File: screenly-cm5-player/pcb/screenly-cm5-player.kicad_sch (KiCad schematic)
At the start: 0 parts

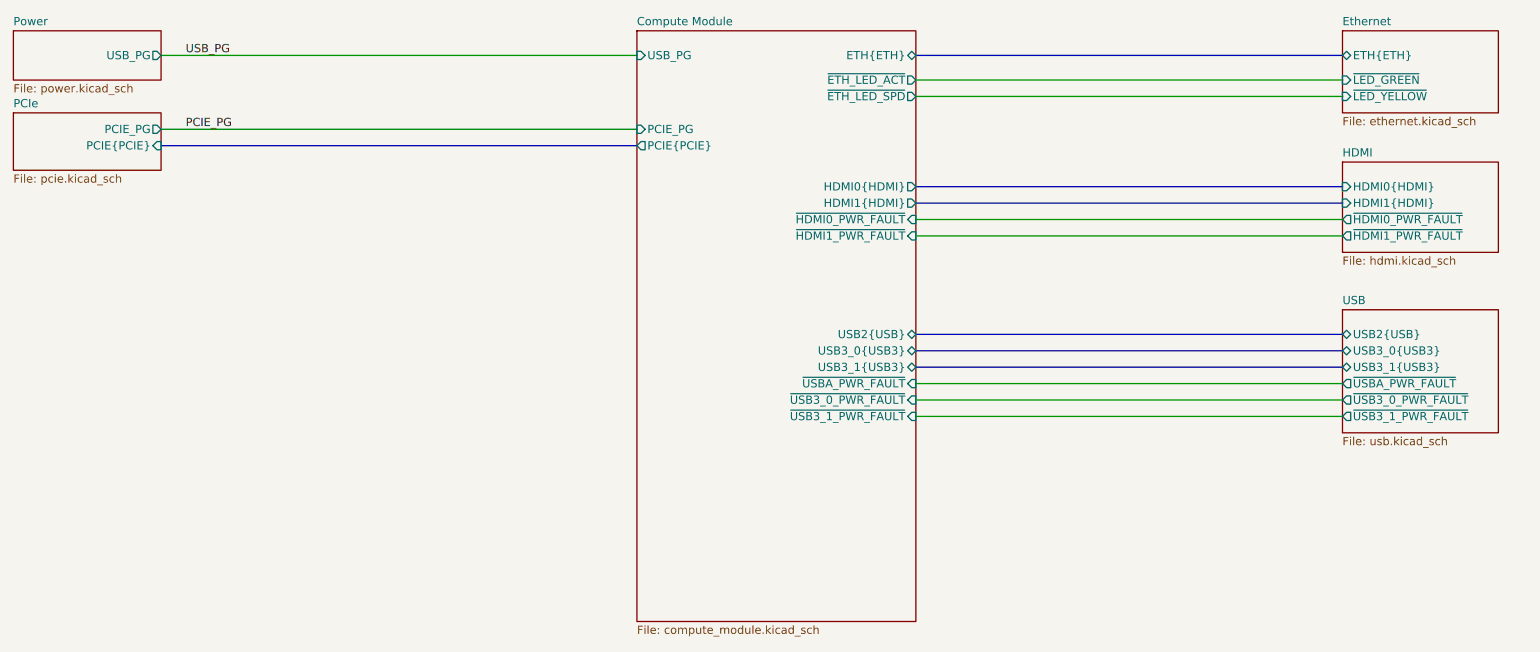
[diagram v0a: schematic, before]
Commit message: Finished USB
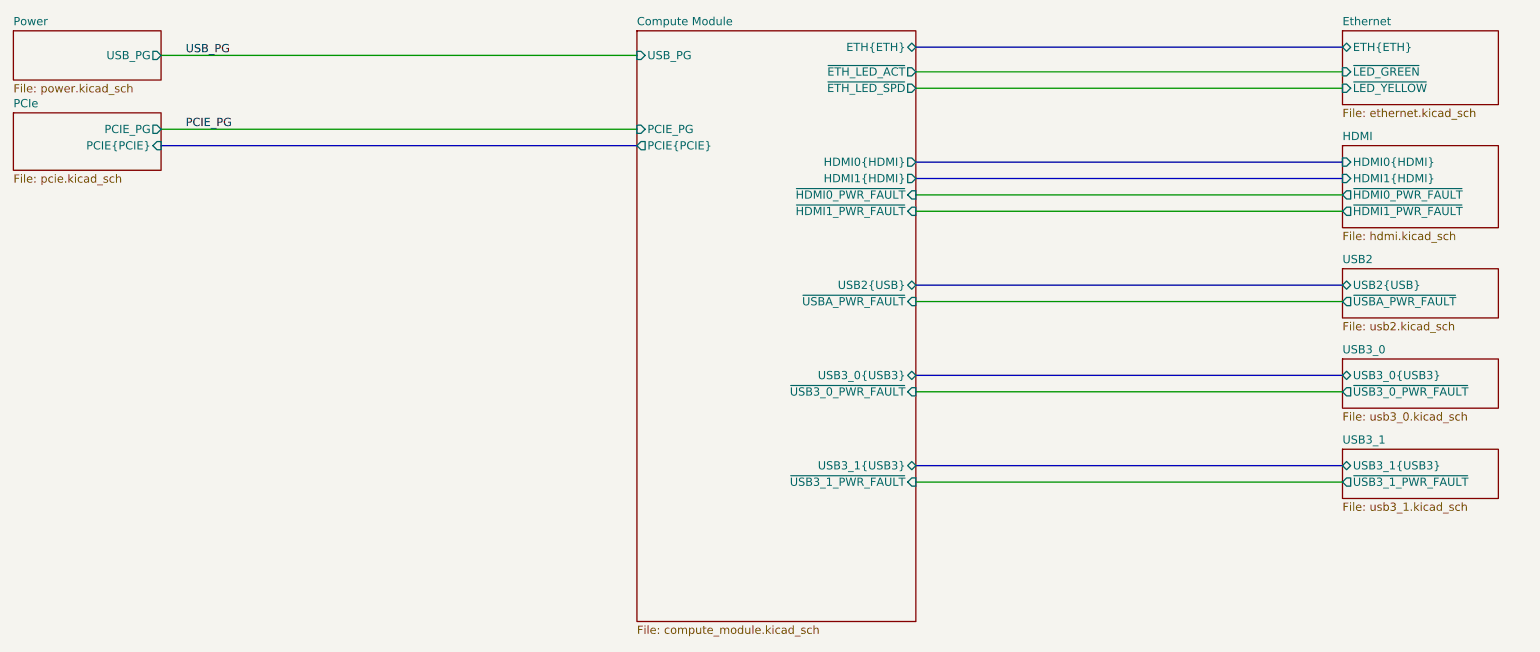
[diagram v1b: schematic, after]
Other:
- sheet USB renamed USB3_0
- added sheet USB2 (usb2.kicad_sch)
- added sheet USB3_1 (usb3_1.kicad_sch)
- sheet USB3_0: file usb.kicad_sch -> usb3_0.kicad_sch
- sheet USB3_0 ports: added none; removed USB2{USB}, USB3_1{USB3}, ~{USB3_1_PWR_FAULT}, ~{USBA_PWR_FAULT}
